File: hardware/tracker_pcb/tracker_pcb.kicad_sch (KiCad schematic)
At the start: 0 parts

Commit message: Parts is parts
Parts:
- added H1, H2, H3, H4: MountingHole_Pad, MountingHole:MountingHole_3mm_Pad_TopBottom, symbol Mechanical:MountingHole_Pad
- added IC1, IC4: DRV8243HQRXYRQ1, footprint:DRV8243HQRXYRQ1, symbol symbol:DRV8243HQRXYRQ1
- added IC2: THVD1426DRLR, footprint:SOTFL50P160X60-8N, symbol symbol:THVD1426DRLR
- added IC3: TPS54302DDCR, SOT95P280X110-6N, symbol symbol:TPS54302DDCR
- added J1, J2, J3: 2601-1102, footprint:CONN2_2601-1102_WAG, symbol symbol:2601-1102
- added RJ1: RJ45 Shielded, footprint:RJ45-TH_R-RJ45R08P-B000, symbol symbol:R-RJ45R08P-B000
- added RJ2: ~, footprint:RJ45-TH_R-RJ45R08P-B000, symbol symbol:R-RJ45R08P-B000
- added U1: ESP32C6_SEEED, footprint:MODULE_113991054, symbol symbol:ESP32C6_SEEED

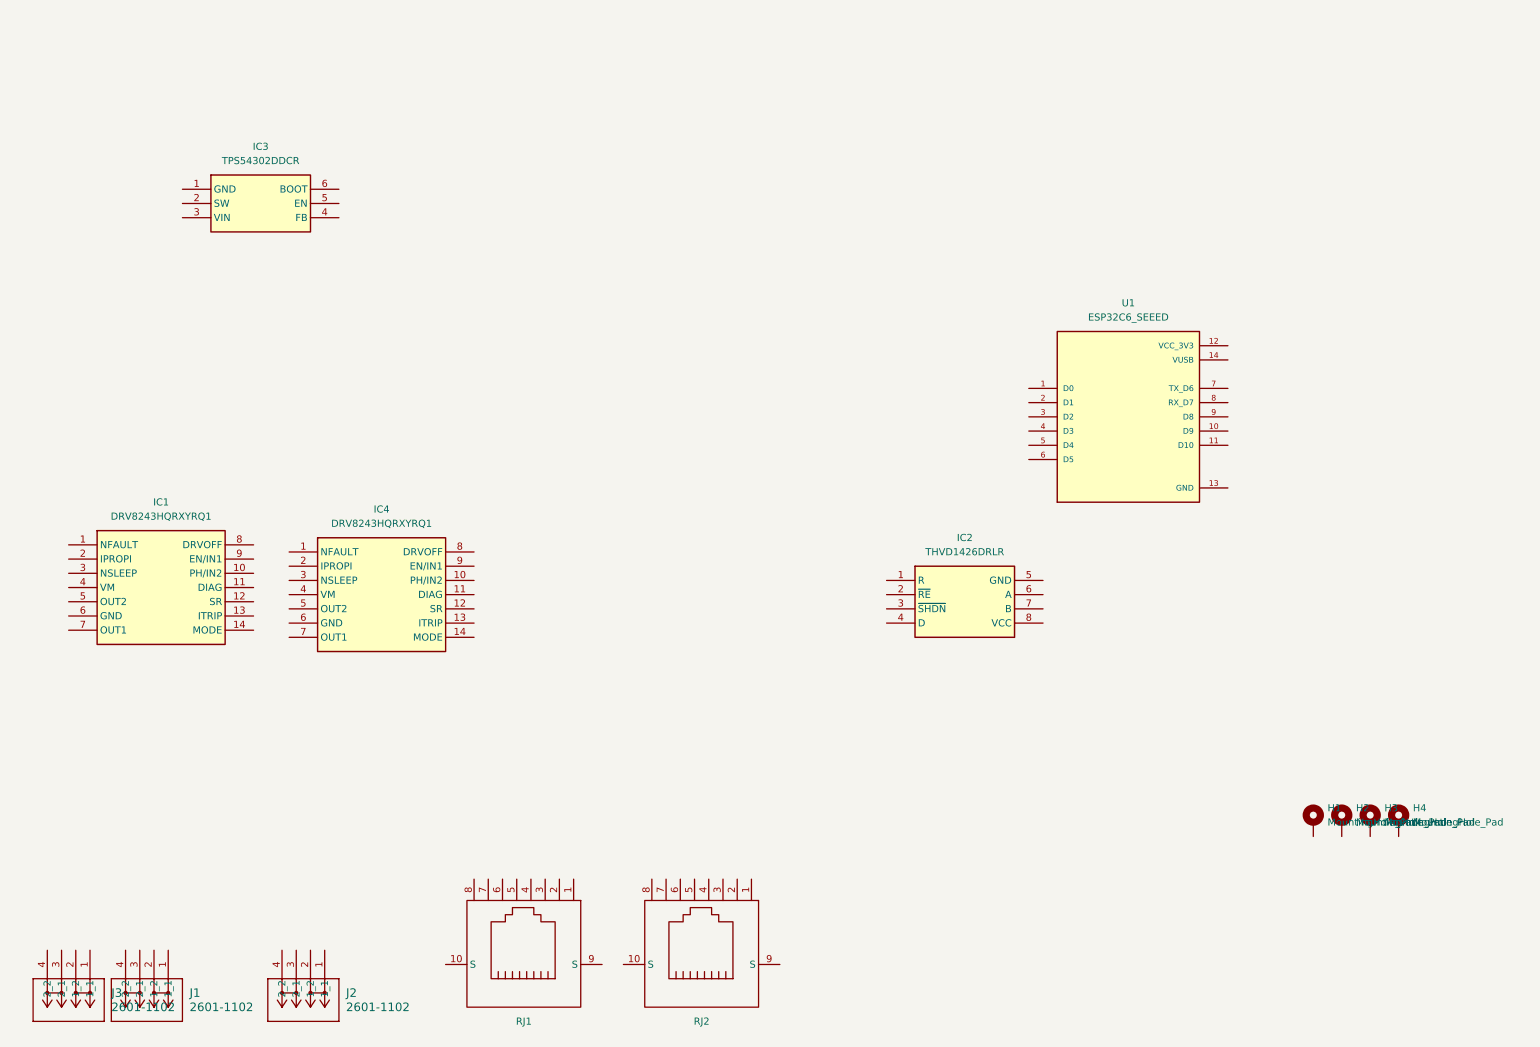
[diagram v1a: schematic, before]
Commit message: WIP
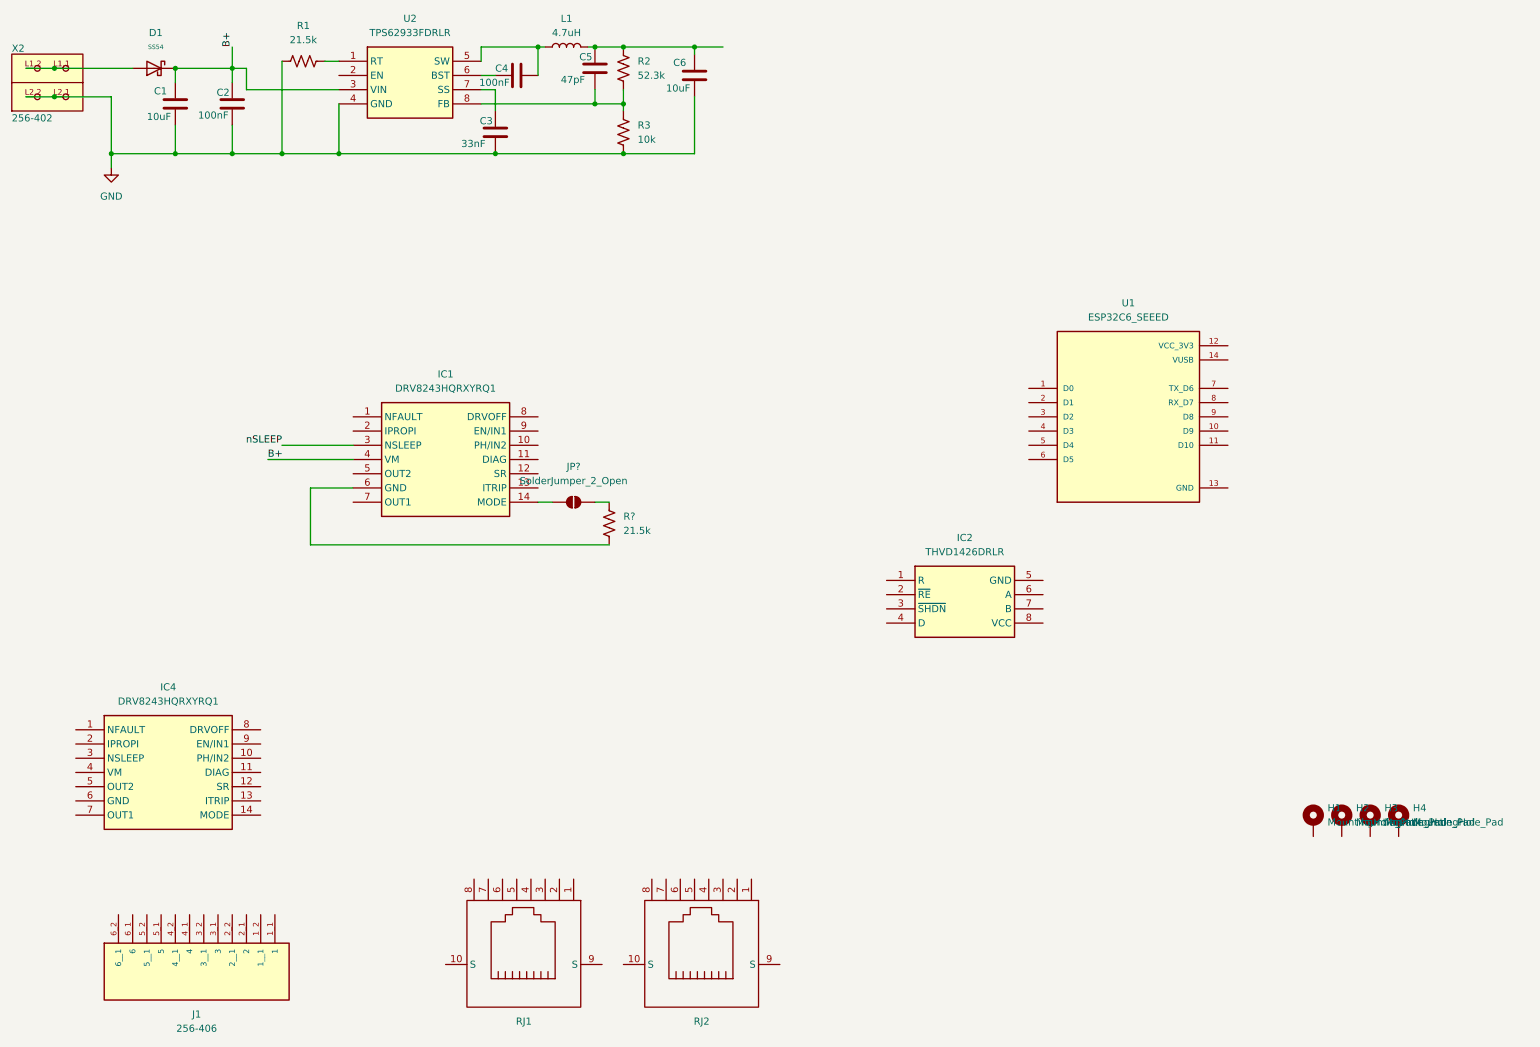
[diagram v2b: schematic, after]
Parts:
- removed IC3: TPS54302DDCR, SOT95P280X110-6N, symbol symbol:TPS54302DDCR
- removed J1, J2, J3: 2601-1102, footprint:CONN2_2601-1102_WAG, symbol symbol:2601-1102
- added C1, C6: 10uF, PCM_JLCPCB:C_1206, symbol Device:C
- added C2, C4: 100nF, PCM_JLCPCB:C_0603, symbol Device:C
- added C3: 33nF, PCM_JLCPCB:C_0603, symbol Device:C
- added C5: 47pF, PCM_JLCPCB:C_0603, symbol Device:C
- added D1: SS54, PCM_JLCPCB:D_SMA, symbol PCM_JLCPCB-Diodes:Schottky,SS54
- added J1: 256-406, footprint:WAGO_256-406, symbol symbol:256-406
- added JP?: SolderJumper_2_Open, symbol Jumper:SolderJumper_2_Open
- added L1: 4.7uH, footprint:IND-SMD_L12.3-W12.3, symbol Device:L
- added R1, R?: 21.5k, PCM_JLCPCB:R_0603, symbol Device:R_US
- added R2: 52.3k, PCM_JLCPCB:R_0603, symbol Device:R_US
- added R3: 10k, PCM_JLCPCB:R_0603, symbol Device:R_US
- added U2: TPS62933FDRLR, footprint:SOTFL50P160X60-8N, symbol symbol:TPS62933FDRLR
- added X2: 256-402, footprint:P-256-402, symbol symbol:256-402
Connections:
- net at IC1.14 (MODE): now also JP?.1 (A)
- net nSLEEP: now reaches IC1.3 (NSLEEP)
- net B+: now reaches IC1.4 (VM)
- net B+: now also C1.1, C2.1, D1.1, U2.3 (VIN)
- net at IC1.6 (GND): now also R?.1
- new net: C5.1, C6.1, L1.2, R2.2
- new net: R1.2, U2.1 (RT)
- new net: C4.2, L1.1, U2.5 (SW)
- new net: C4.1, U2.6 (BST)
- new net: C3.1, U2.7 (SS)
- new net: C5.2, R2.1, R3.2, U2.8 (FB)
- new net: JP?.2 (B), R?.2
- new net: D1.2, X2.L1.1, X2.L1.2
- new net GND: C1.2, C2.2, C3.2, C6.2, R1.1, R3.1, U2.4 (GND), X2.L2.1, X2.L2.2
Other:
- moved on the sheet: IC1, IC4
